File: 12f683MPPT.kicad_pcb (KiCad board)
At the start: 2 copper layers, 98.3 x 72.6 mm, 58 parts, among them J1 Conn_01x01_Male, J2 Conn_01x01_Male, J3 Conn_01x01_Male, J4 Conn_01x01_Male, J5 Vin, J6 GND, J7 12V, Q1 BUK9511-55A127, Q2 BUK9511-55A127, Q3 2N2222A, Q4 2N2222A, Q5 2N2907A, SW1 SW_Push, U1 LM7805_TO220, U2 PIC12F683-IP, U3 LM358

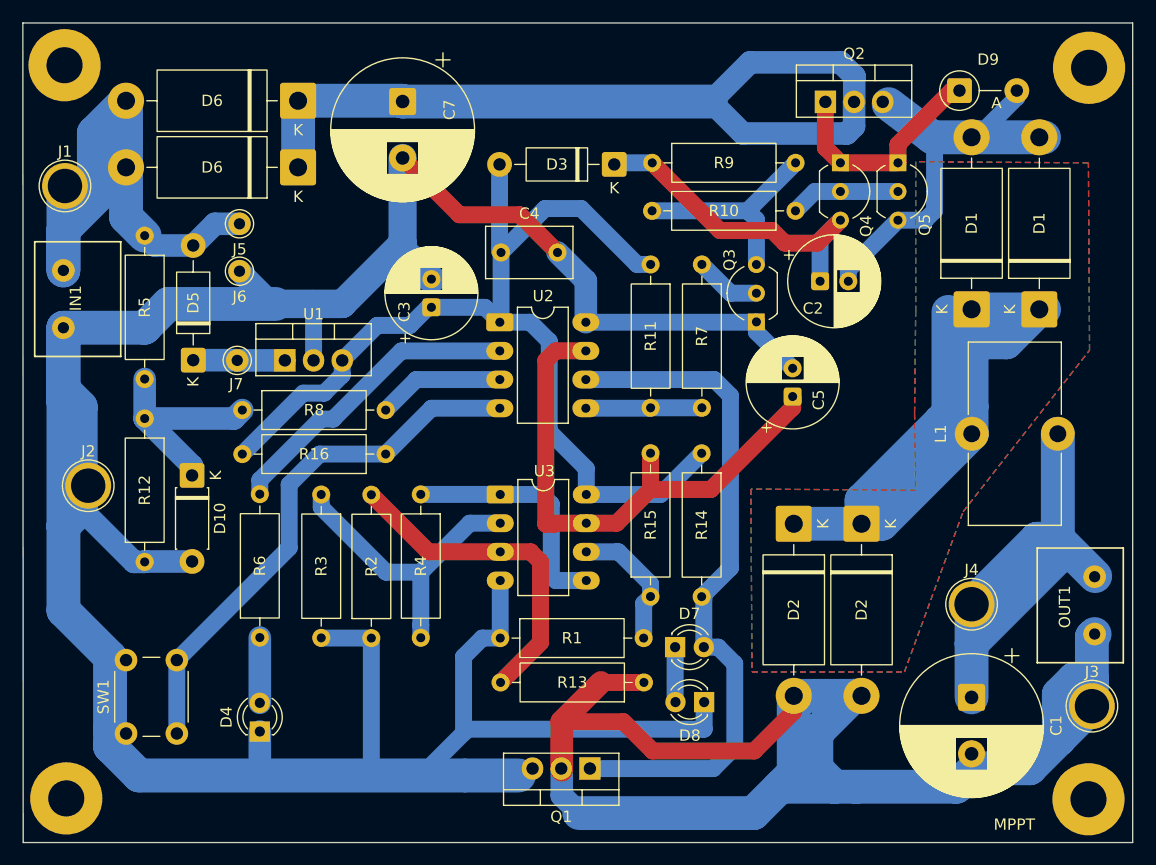
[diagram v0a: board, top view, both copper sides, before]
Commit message: Update PCB files.
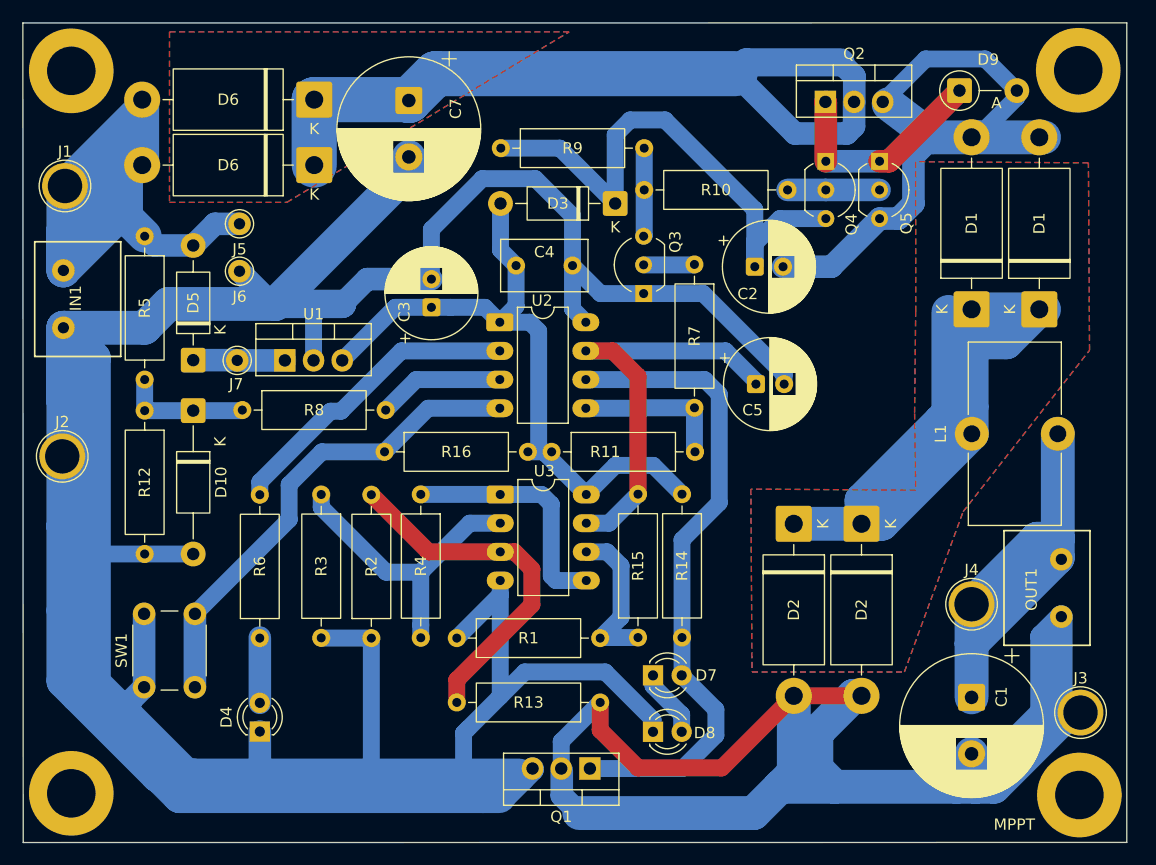
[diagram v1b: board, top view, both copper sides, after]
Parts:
- D10: footprint Diode_THT:D_DO-41_SOD81_P7.62mm_Horizontal -> Diode_THT:D_DO-41_SOD81_P12.70mm_Horizontal
- REF** (x4): value MountingHole_3.2mm_M3_Pad -> MountingHole_4.3mm_M4_DIN965_Pad; footprint MountingHole:MountingHole_3.2mm_M3_Pad -> MountingHole:MountingHole_4.3mm_M4_DIN965_Pad
- moved R11 18.8 mm to (83.0, 64.5), turned to 0 degrees
- moved R9 13.5 mm to (78.5, 37.6)
- moved Q3 10.3 mm to (91.2, 50.5)
- moved C2 5.93 mm to (101.0, 48.1)
- moved D10 5.74 mm to (51.3, 60.9)
- moved D8 5.24 mm to (92.0, 89.3), turned to 0 degrees
- moved SW1 4.40 mm to (47.0, 85.3)
- moved R13 4.26 mm to (87.3, 86.7)
- moved R14 4.02 mm to (94.6, 68.2)
- moved R1 3.85 mm to (74.7, 81.0)
- moved R15 3.80 mm to (90.7, 81.0)
- moved J2 3.47 mm to (39.7, 64.9)
- moved D3 3.46 mm to (88.7, 42.5)
- moved C5 3.43 mm to (101.1, 58.5), turned to 0 degrees
- moved OUT1 3.33 mm to (128.2, 79.1)
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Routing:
- net GNDPWR: track 314.3 -> 406.2 mm
- net Net-(D3-A): track 92.4 -> 59.3 mm
- net /BootStrap: track 30.2 -> 51.1 mm
- net Net-(D1-A): track 38.5 -> 55.5 mm
- net Net-(Q3-C): track 19.6 -> 7.82 mm
- net /PV-Current: track 48.8 -> 38.1 mm
- net +24V: track 48.5 -> 58.5 mm
- net PRI_LO: track 130.9 -> 139.0 mm
- net Net-(D10-K): track 19.2 -> 11.4 mm
- net Net-(U2-GP3): track 47.6 -> 42.9 mm
- net PRI_HI: track 44.7 -> 40.1 mm
- net /3.6v: track 61.0 -> 57.6 mm
- net Net-(U2-GP2): track 10.3 -> 13.6 mm
- net Net-(D6-K): track 75.8 -> 73.2 mm
- net Net-(U3B--): track 11.9 -> 14.1 mm
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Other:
- board size 98.3 x 72.6 mm -> 97.8 x 72.6 mm
- board text added: "K"
